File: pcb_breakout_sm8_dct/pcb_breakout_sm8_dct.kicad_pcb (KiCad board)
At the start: 2 copper layers, 2 parts, among them J1 Conn_02x04_Counter_Clockwise, J2 Conn_02x04_Counter_Clockwise

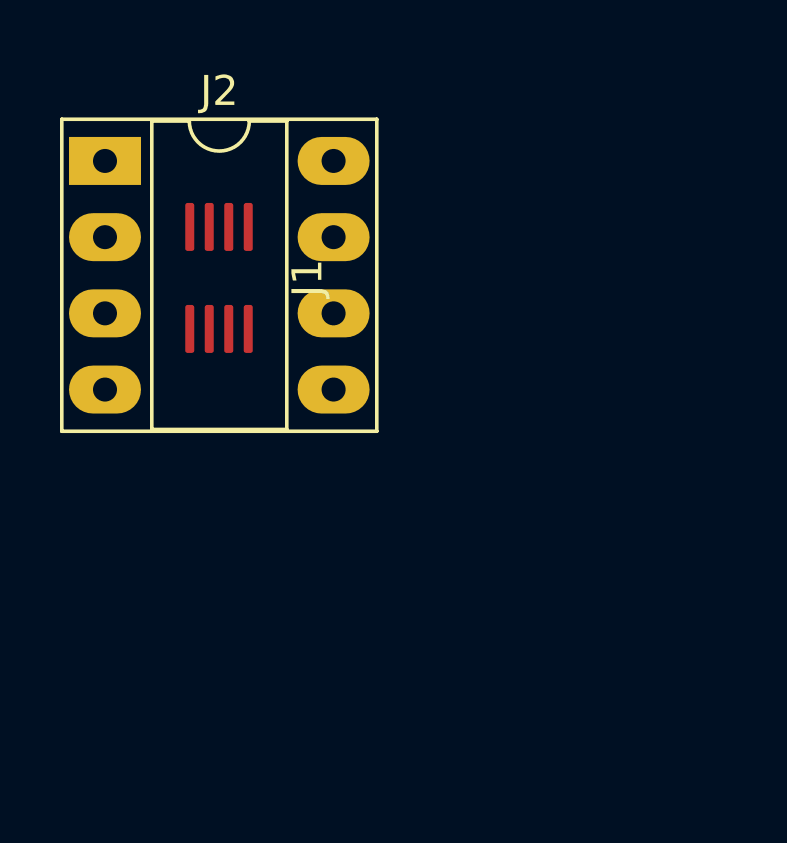
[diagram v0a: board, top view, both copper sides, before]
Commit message: dct us8 breakout
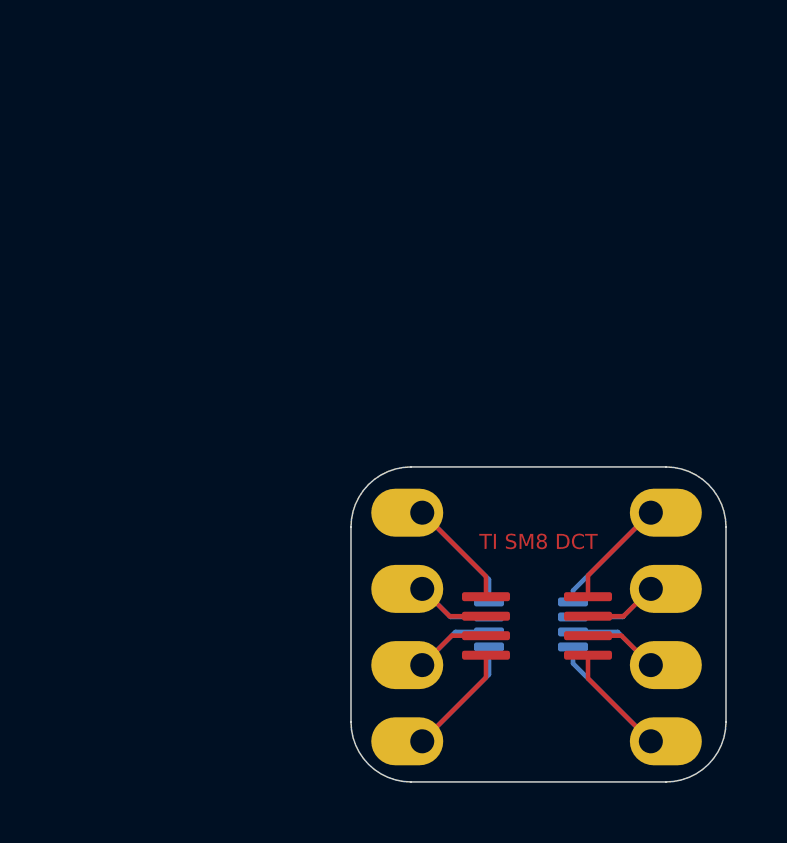
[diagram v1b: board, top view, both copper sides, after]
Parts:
- added REF**: OnSemi_US8-8, Packages:OnSemi_US8-8, B.Cu at (156.0, 94.2)
- moved J2 15.8 mm to (152.4, 90.5)
- moved J1 15.7 mm to (156.2, 94.3), turned to 0 degrees
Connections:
- J2 pad 1: Net-(J2-Pad1) -> Net-(J1-Pad1)
- J2 pad 2: Net-(J2-Pad2) -> Net-(J1-Pad2)
- J2 pad 3: Net-(J2-Pad3) -> Net-(J1-Pad3)
- J2 pad 4: Net-(J2-Pad4) -> Net-(J1-Pad4)
- J2 pad 5: Net-(J2-Pad5) -> Net-(J1-Pad5)
- J2 pad 6: Net-(J2-Pad6) -> Net-(J1-Pad6)
- J2 pad 7: Net-(J2-Pad7) -> Net-(J1-Pad7)
- J2 pad 8: Net-(J2-Pad8) -> Net-(J1-Pad8)
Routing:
- net Net-(J1-Pad5): track 0.00 -> 7.96 mm
- net Net-(J1-Pad4): track 0.00 -> 7.82 mm
- net Net-(J1-Pad8): track 0.00 -> 7.72 mm
- net Net-(J1-Pad1): track 0.00 -> 7.58 mm
- net Net-(J1-Pad6): track 0.00 -> 5.55 mm
- net Net-(J1-Pad7): track 0.00 -> 5.45 mm
- net Net-(J1-Pad3): track 0.00 -> 5.21 mm
- net Net-(J1-Pad2): track 0.00 -> 5.11 mm
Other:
- board outline added: 12.5 x 10.5 mm
- net class 6/6 added: clearance 0.1524, trace_width 0.1524, via_dia 0.8, via_drill 0.4
- rule trace_min: 0.2 -> 0.1524
- board text added: "OnSemi US8"
- board text added: "TI SM8 DCT"
